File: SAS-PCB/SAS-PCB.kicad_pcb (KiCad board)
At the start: 2 copper layers, 96.5 x 85.5 mm, 23 parts, among them J1_Batt1 691137710002, J2-LCD1 Conn_01x04_Socket, J3-LCD2 Conn_01x04_Socket, J4-BMP280 Conn_01x06_Pin, J5-GPS1 Conn_01x04_Socket, J6-cable-plat1 Conn_02x20_Odd_Even, J7-RFD900x1 691137710002, J8-Fan1 Conn_01x04_Socket, J9-Fan2 Conn_01x04_Socket

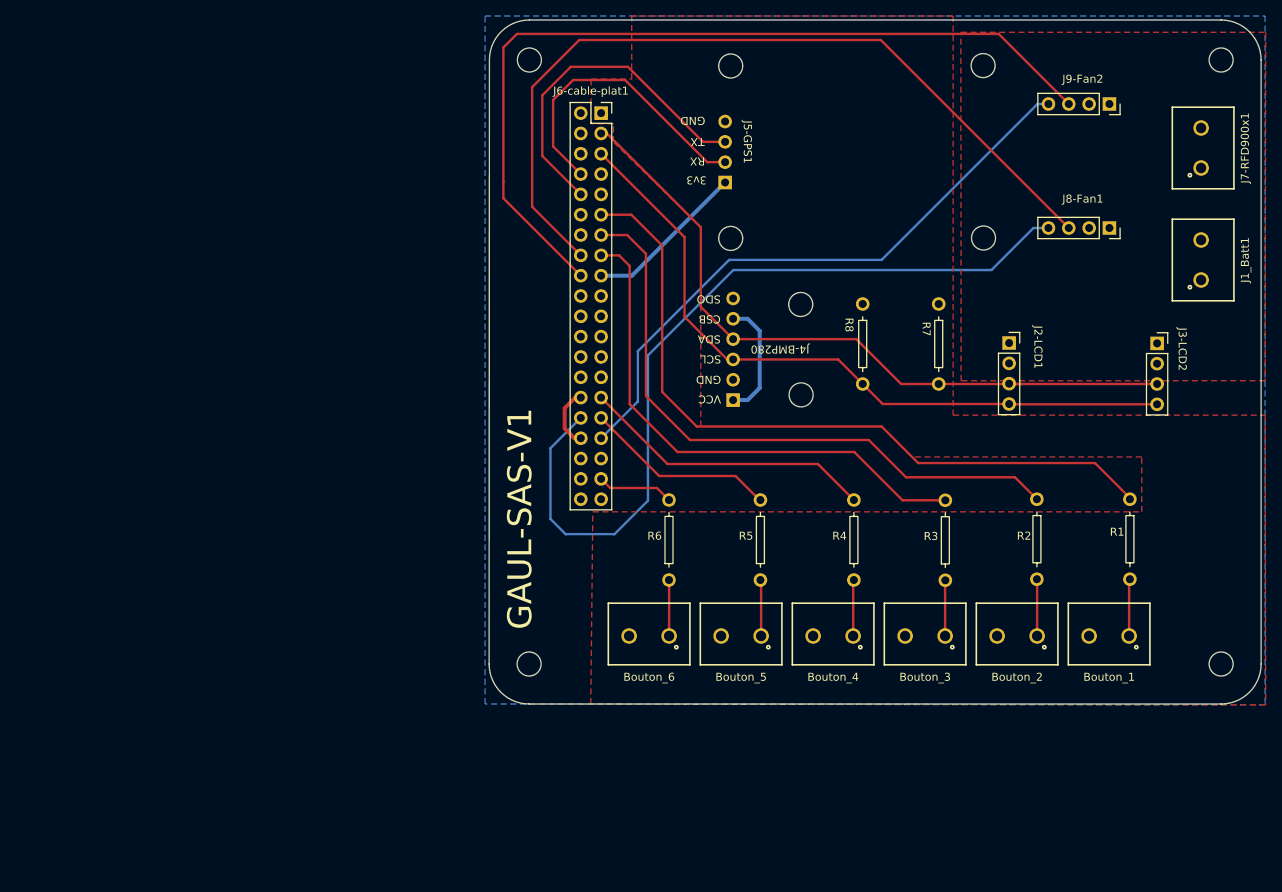
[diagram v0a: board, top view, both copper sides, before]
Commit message: u1
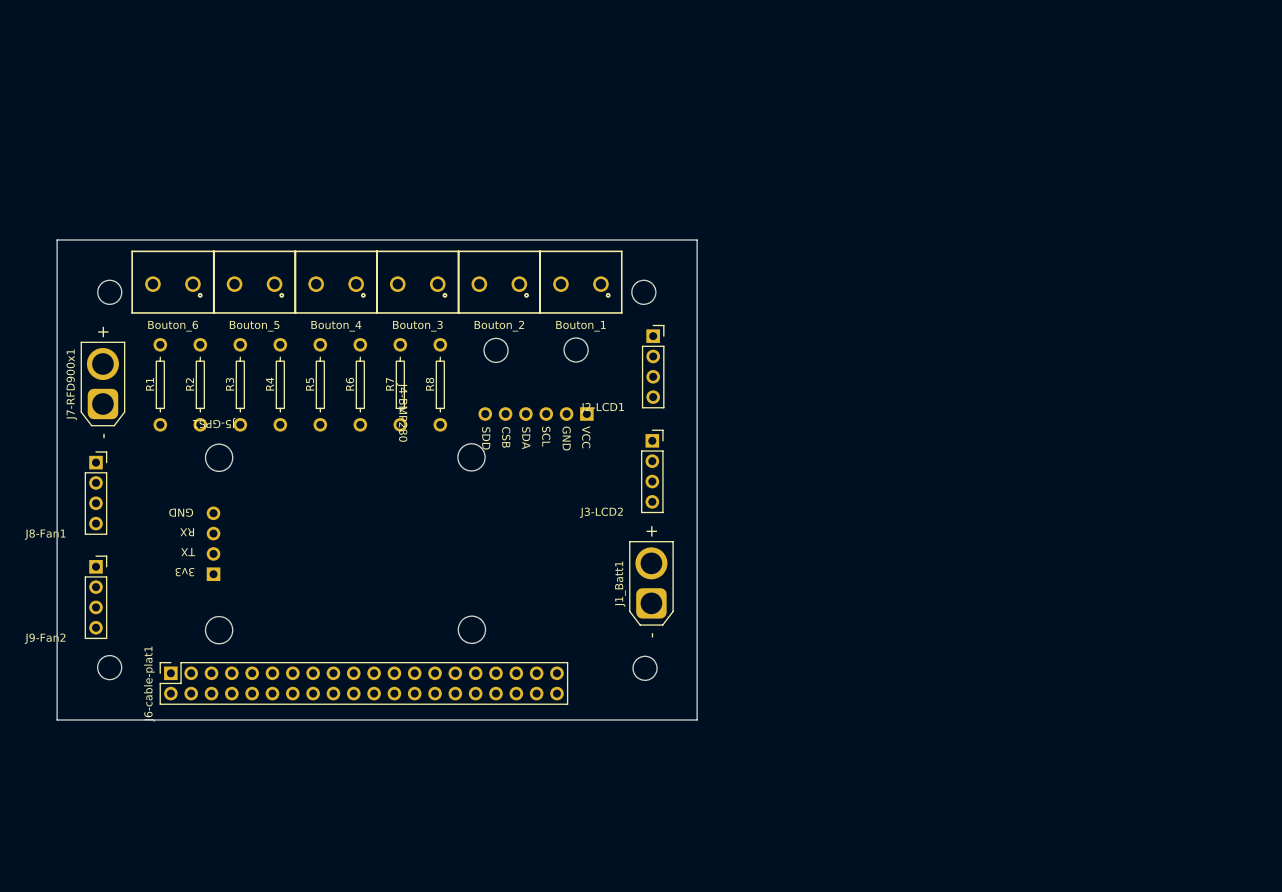
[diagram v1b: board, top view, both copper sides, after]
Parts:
- J1_Batt1, J7-RFD900x1: footprint SAS-Librarie-Empreinte:bornie_2position -> SAS-Librarie-Empreinte:AMASS_XT30U-F_1x02_P5.0mm_Vertical
- moved J9-Fan2 143.7 mm to (58.6, 110.2), turned to 0 degrees
- moved J7-RFD900x1 141.0 mm to (65.7, 80.5)
- moved J8-Fan1 131.5 mm to (58.6, 97.2), turned to 0 degrees
- moved R1 122.6 mm to (73.0, 78.0), turned to 90 degrees
- moved R2 106.2 mm to (78.0, 78.0), turned to 90 degrees
- moved R3 96.2 mm to (83.0, 78.0)
- moved J6-cable-plat1 88.3 mm to (74.2, 114.2), turned to 90 degrees
- moved J1_Batt1 81.0 mm to (134.3, 105.4)
- moved J5-GPS1 80.5 mm to (79.5, 98.0)
- moved R4 80.4 mm to (88.0, 78.0)
- moved Bouton_1 79.3 mm to (125.5, 65.5)
- moved Bouton_2 78.2 mm to (115.3, 65.5)
- moved Bouton_3 77.2 mm to (105.1, 65.5)
- moved Bouton_4 76.1 mm to (94.9, 65.5)
- moved Bouton_5 75.1 mm to (84.7, 65.5)
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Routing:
- net Fan2_RPM: track 107.5 -> 0.00 mm
- net Fan1_PWM: track 103.7 -> 0.00 mm
- net Fan1_RPM: track 102.8 -> 0.00 mm
- net Bouton_1: track 91.6 -> 0.00 mm
- net SDA: track 89.8 -> 0.00 mm
- net SCL: track 88.4 -> 0.00 mm
- net Bouton_2: track 78.7 -> 0.00 mm
- net Fan2_PWM: track 76.9 -> 0.00 mm
- net Bouton_3: track 65.8 -> 0.00 mm
- net RXD: track 42.6 -> 0.00 mm
- net TXD: track 37.5 -> 0.00 mm
- net Bouton_4: track 36.8 -> 0.00 mm
- net +3.3V: track 35.4 -> 0.00 mm
- net Bouton_5: track 24.0 -> 0.00 mm
- net Bouton_6: track 9.58 -> 0.00 mm
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- removed copper zone on F.Cu, net +3.3V
- removed copper zone on F.Cu, net +5V
- removed copper zone on B.Cu, net GND
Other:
- board size 96.5 x 85.5 mm -> 80 x 60 mm
- board text removed: "GAUL-SAS-V1"

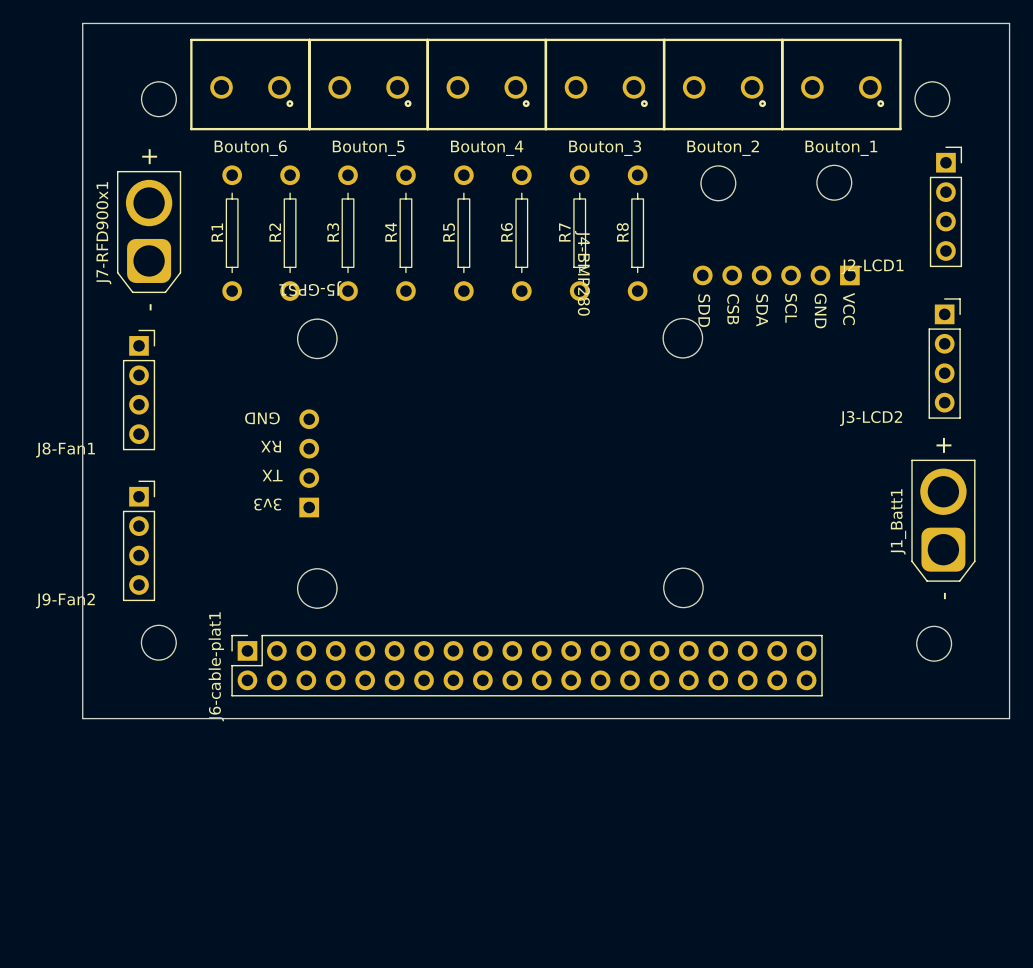
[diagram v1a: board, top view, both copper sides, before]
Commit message: U2
trial 2
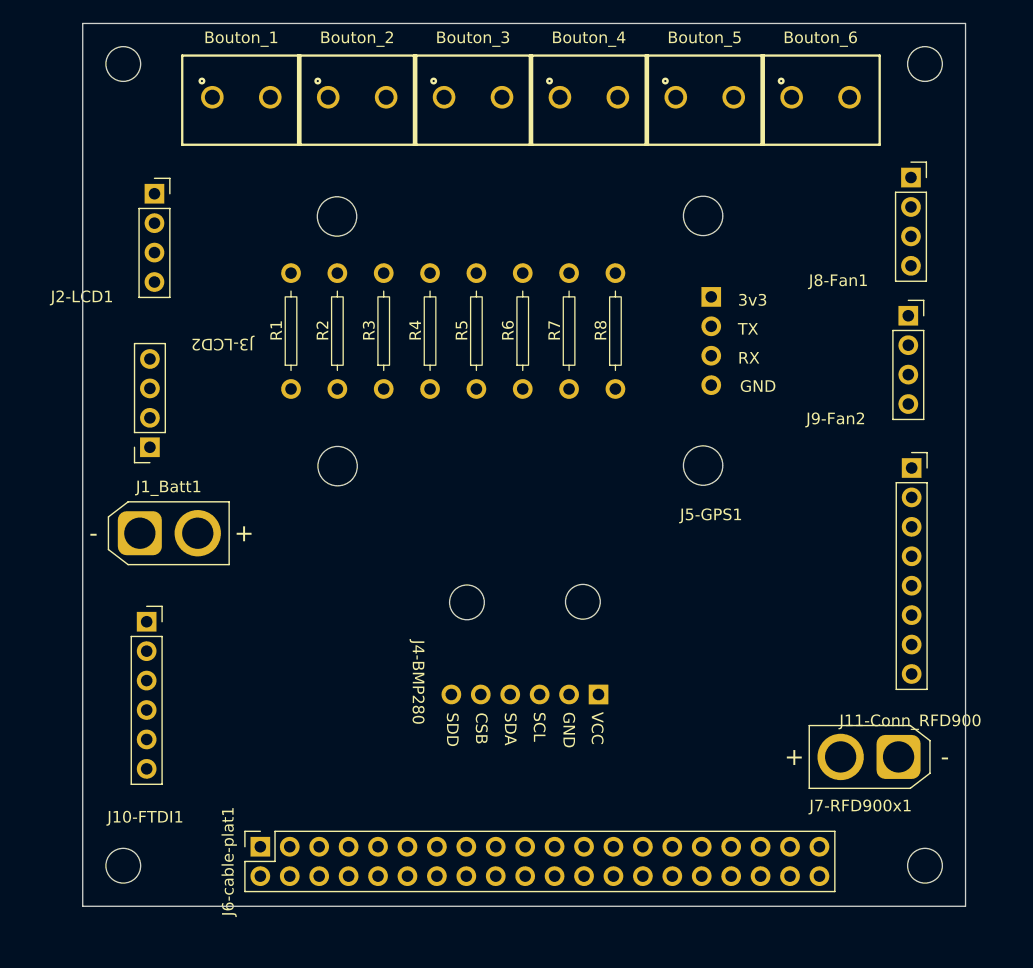
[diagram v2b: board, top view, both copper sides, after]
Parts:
- added J10-FTDI1: Conn_01x06, SAS-Librarie-Empreinte:Conn_6_pos, F.Cu at (65.4, 129.0)
- added J11-Conn_RFD900: Conn_01x08, SAS-Librarie-Empreinte:Conn_8_pos, F.Cu at (131.4, 120.7)
- moved J7-RFD900x1 77.6 mm to (130.4, 123.3), turned to 180 degrees
- moved J1_Batt1 69.4 mm to (64.9, 104.0), turned to 0 degrees
- moved J2-LCD1 68.4 mm to (59.9, 84.1)
- moved J9-Fan2 68.2 mm to (125.0, 94.6)
- moved J8-Fan1 68.2 mm to (125.2, 82.7)
- moved J3-LCD2 56.6 mm to (72.0, 87.2), turned to 180 degrees
- moved Bouton_1 51.8 mm to (73.7, 66.4), turned to 0 degrees
- moved Bouton_6 49.2 mm to (123.7, 66.4), turned to 0 degrees
- moved J4-BMP280 42.2 mm to (91.8, 117.9)
- moved J5-GPS1 36.3 mm to (114.2, 87.4), turned to 0 degrees
- moved Bouton_2 31.6 mm to (83.7, 66.4), turned to 0 degrees
- moved Bouton_5 29.0 mm to (113.7, 66.4), turned to 0 degrees
- moved J6-cable-plat1 16.9 mm to (75.3, 131.1)
- moved Bouton_3 11.4 mm to (93.7, 66.4), turned to 0 degrees
- moved R1 9.86 mm to (78.1, 86.5)
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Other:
- board size 80 x 60 mm -> 76.2 x 76.2 mm

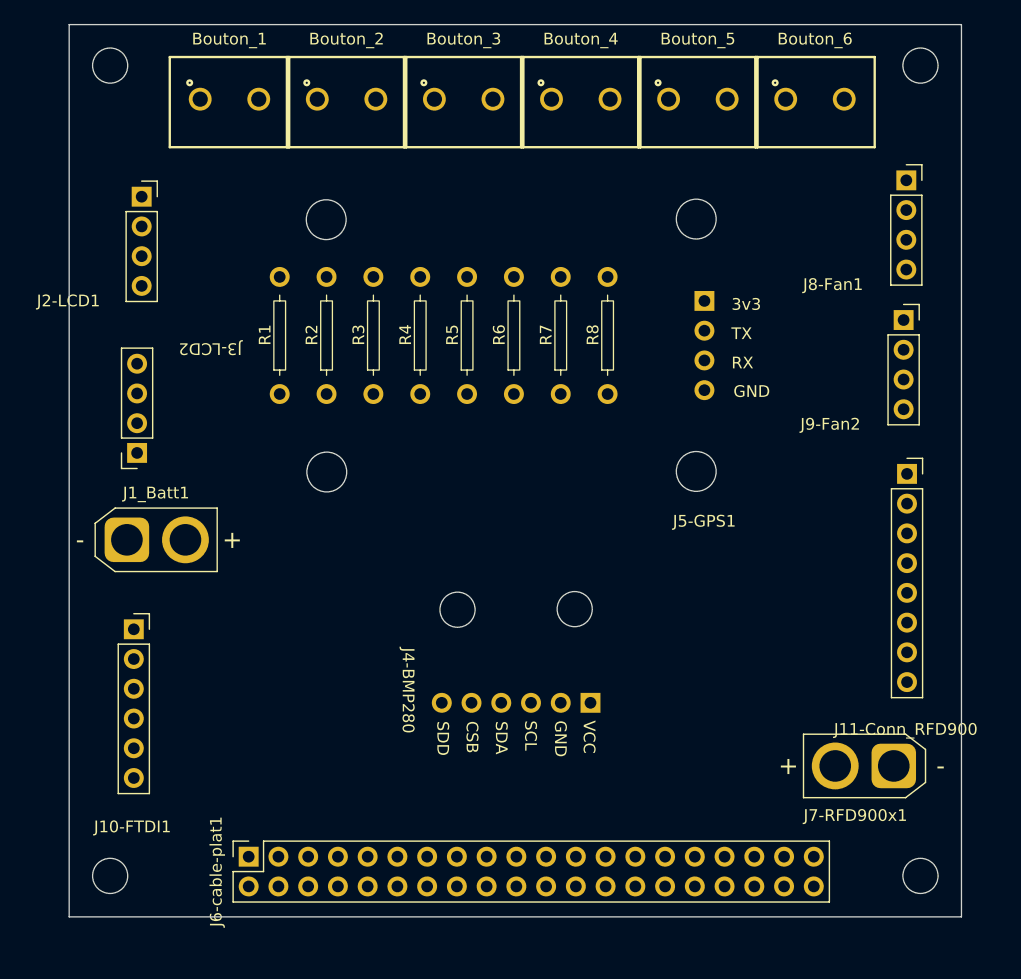
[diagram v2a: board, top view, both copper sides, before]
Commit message: Version_a_amiliorer
pas tant fonctionnel
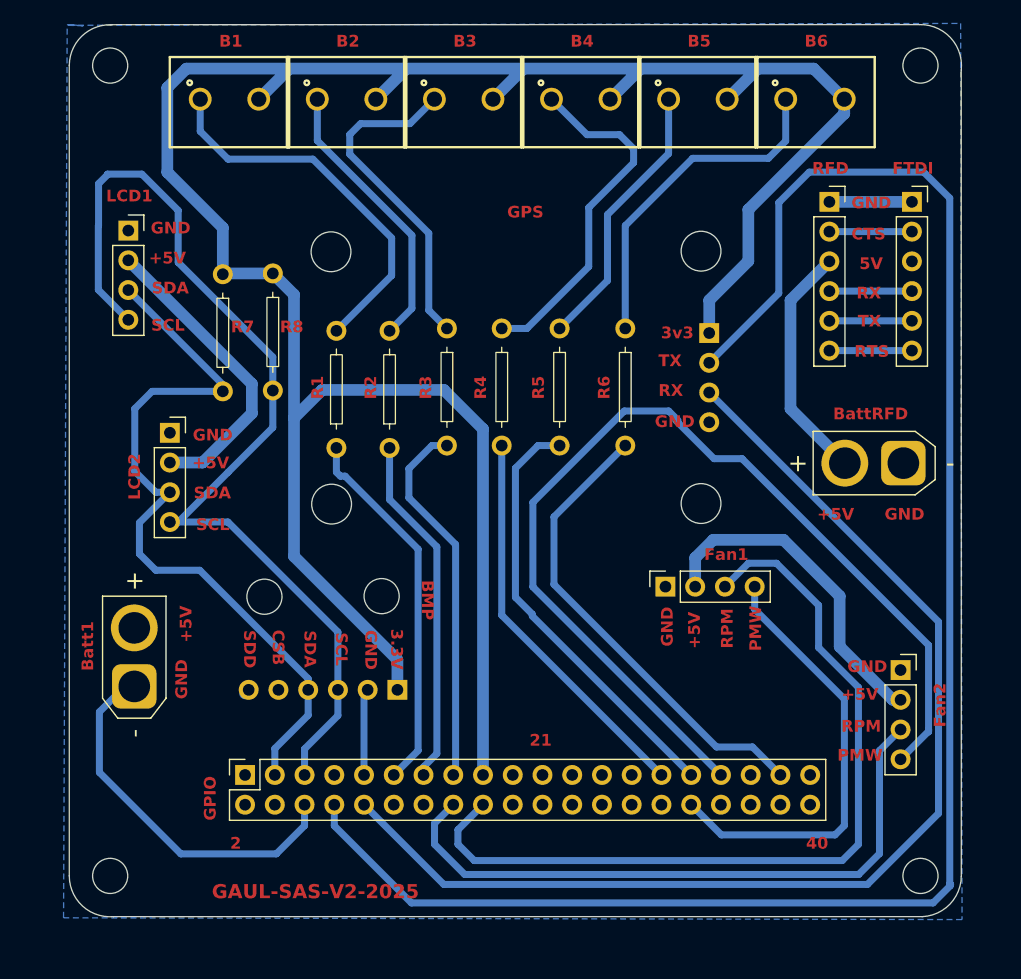
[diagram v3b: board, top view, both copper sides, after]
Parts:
- removed J11-Conn_RFD900: Conn_01x08, SAS-Librarie-Empreinte:Conn_8_pos
- added J10-FTDI2: Conn_01x06, SAS-Librarie-Empreinte:Conn_6_pos, F.Cu at (124.8, 92.5)
- moved J10-FTDI1 75.8 mm to (131.9, 92.5)
- moved J8-Fan1 31.9 mm to (120.3, 114.2), turned to 90 degrees
- moved J9-Fan2 29.9 mm to (124.8, 124.5)
- moved R7 29.1 mm to (73.0, 86.4), turned to -90 degrees
- moved R8 28.8 mm to (77.3, 86.3), turned to -90 degrees
- moved J7-RFD900x1 25.9 mm to (131.2, 97.5)
- moved J3-LCD2 19.6 mm to (62.4, 104.3), turned to 0 degrees
- moved J4-BMP280 16.5 mm to (75.3, 116.8)
- moved J1_Batt1 12.5 mm to (65.6, 116.5), turned to 90 degrees
- moved R6 10.4 mm to (107.4, 91.0), turned to -90 degrees
- moved R5 8.97 mm to (101.8, 91.0), turned to -90 degrees
- moved R4 8.18 mm to (96.8, 91.0), turned to -90 degrees
- moved R3 7.62 mm to (92.2, 91.0), turned to -90 degrees
- moved R2 7.08 mm to (87.5, 91.0)
- moved J6-cable-plat1 6.99 mm to (75.0, 124.1)
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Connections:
- J10-FTDI1 pad 3: +5V -> unconnected-(J10-FTDI1-Pin_3-Pad3)
- J10-FTDI1 pad 4: RFD_TX -> RFD_RX
- J10-FTDI1 pad 5: RFD_RX -> RFD_TX
- J6-cable-plat1 pad 16: Fan1_RPM -> Fan2_RPM
- J6-cable-plat1 pad 18: Fan2_RPM -> Fan1_RPM
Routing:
- net +3.3V: track 0.00 -> 213.5 mm
- net TXD: track 0.00 -> 149.4 mm
- net RXD: track 0.00 -> 98.4 mm
- net SCL: track 0.00 -> 86.8 mm
- net Fan2_PWM: track 0.00 -> 86.4 mm
- net +5V: track 0.00 -> 75.9 mm
- net Fan1_RPM: track 0.00 -> 71.8 mm
- net SDA: track 0.00 -> 63.9 mm
- net Fan2_RPM: track 0.00 -> 55.2 mm
- net GND: track 0.00 -> 46.7 mm
- net Bouton_6: track 0.00 -> 40.5 mm
- net Fan1_PWM: track 0.00 -> 38.1 mm
- net Bouton_5: track 0.00 -> 37.0 mm
- net Bouton_4: track 0.00 -> 33.8 mm
- net Net-(Bouton_1-GND): track 0.00 -> 32.7 mm
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- added copper zone on B.Cu, net GND
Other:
- outline, holes or cut-outs redrawn
- board text added: "+5V"
- board text added: "2"
- board text added: "21"
- board text added: "3.3V"
- board text added: "3v3"
- board text added: "40"
- board text added: "5V"
- board text added: "B1"
- board text added: "B2"
- board text added: "B3"
- board text added: "B4"
- board text added: "B5"
- board text added: "B6"
- board text added: "BMP"
- board text added: "Batt1"
- board text added: "BattRFD"
- board text added: "CSB"
- board text added: "CTS"
- board text added: "FTDI"
- board text added: "Fan1"
- board text added: "Fan2"
- board text added: "GAUL-SAS-V2-2025"
- board text added: "GND"
- board text added: "GPIO"
- board text added: "GPS"
- board text added: "LCD1"
- board text added: "LCD2"
- board text added: "PMW"
- board text added: "R1"
- board text added: "R2"
- board text added: "R3"
- board text added: "R4"
- board text added: "R5"
- board text added: "R6"
- board text added: "R7"
- board text added: "R8"
- board text added: "RFD"
- board text added: "RPM"
- board text added: "RTS"
- board text added: "RX"
- board text added: "SCL"
- board text added: "SDA"
- board text added: "SDD"
- board text added: "TX"
